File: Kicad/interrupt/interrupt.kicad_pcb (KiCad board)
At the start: 2 copper layers, 68.6 x 53.3 mm, 30 parts, among them IC1 LTC1050CS8#PBF, J1 Conn_LORA, P1 Power, P2 Analog, P3 Digital, P4 Digital, P5 CONN_01X01, P6 CONN_01X01, P7 CONN_01X01, P8 CONN_01X01, Q1 IRF520, U1 GAZ_TO_5

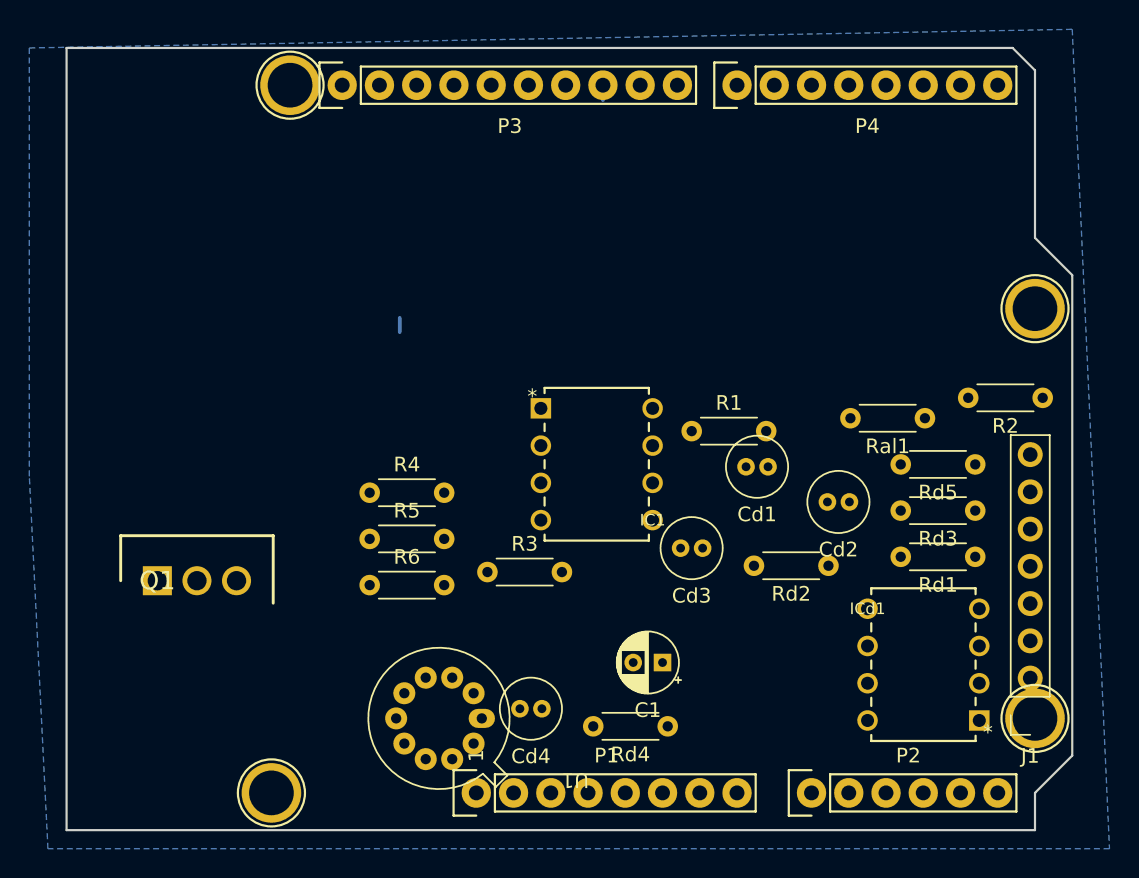
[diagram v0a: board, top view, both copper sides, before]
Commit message: maj
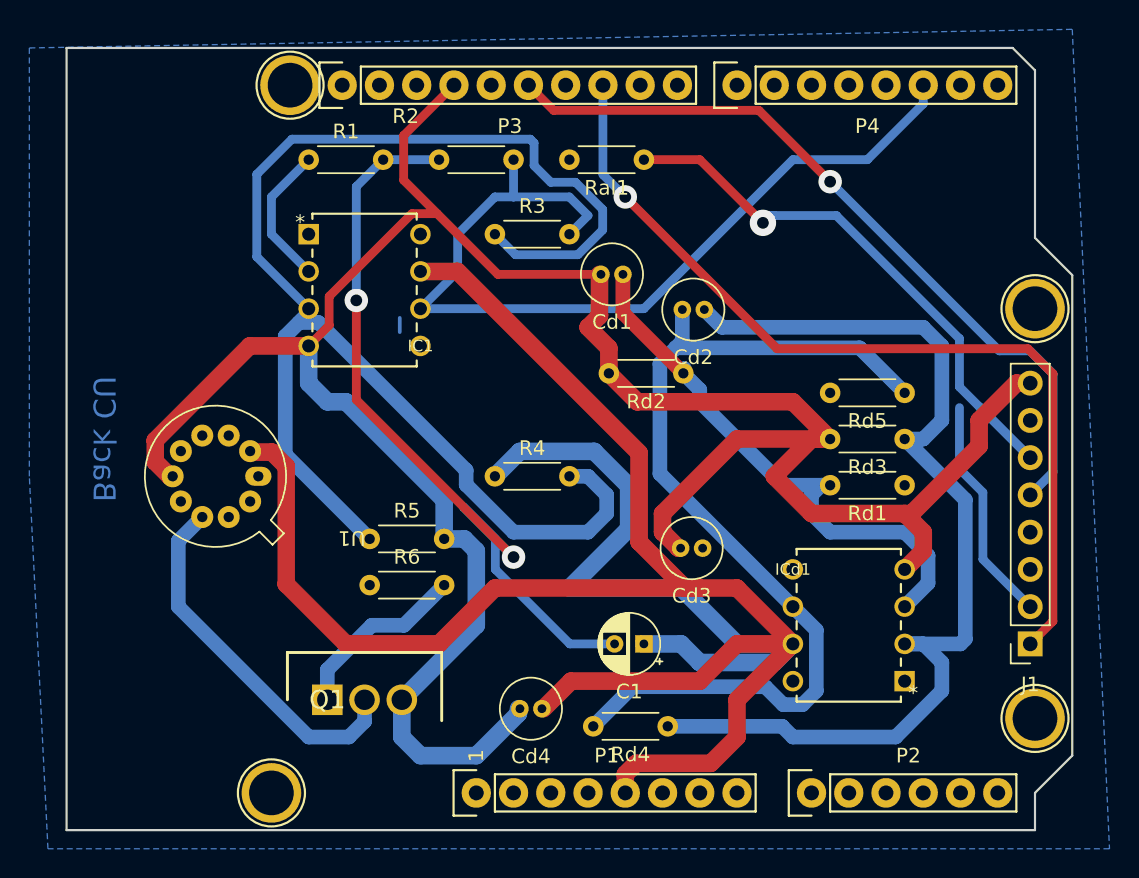
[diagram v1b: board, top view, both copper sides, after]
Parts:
- Q1: footprint IRF520:TO270P460X1020X2008-3P -> KiCadIRF:TO254P465X1024X2050-3P
- moved R2 39.6 mm to (141.5, 80.6)
- moved R1 32.0 mm to (127.5, 80.6)
- moved Ral1 26.0 mm to (150.4, 80.6)
- moved R3 23.0 mm to (140.2, 85.7)
- moved U1 22.5 mm to (122.8, 101.4)
- moved IC1 19.8 mm to (135.1, 93.3)
- moved Cd2 16.4 mm to (154.5, 90.9)
- moved Cd1 16.4 mm to (148.9, 88.5)
- moved Rd2 16.4 mm to (153.1, 95.2)
- moved Q1 14.2 mm to (128.8, 117.5)
- moved R4 8.61 mm to (140.2, 102.2)
- moved Rd3 6.86 mm to (168.1, 99.7)
- moved Rd1 6.86 mm to (168.1, 102.8)
- moved Rd5 6.86 mm to (168.1, 96.5)
- moved ICd1 5.75 mm to (160.5, 108.6)
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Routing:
- net GND: track 0.00 -> 172.8 mm
- net +5V: track 0.00 -> 166.8 mm
- net Net-(IC1-Pad3): track 0.00 -> 99.2 mm
- net Net-(Cd2-Pad1): track 0.00 -> 70.3 mm
- net Net-(Cd2-Pad2): track 0.00 -> 65.2 mm
- net /VAOP: track 0.00 -> 62.3 mm
- net /TX: track 1.99 -> 61.5 mm, vias 0 -> 1
- net Net-(C1-Pad2): track 0.00 -> 56.4 mm, vias 0 -> 2
- net /RST: track 0.00 -> 52.8 mm, vias 0 -> 1
- net +3V3: track 0.00 -> 42.0 mm, vias 0 -> 1
- net Net-(Cd1-Pad1): track 0.00 -> 38.6 mm
- net /GND_Gaz: track 0.00 -> 25.1 mm
- net /RX: track 0.00 -> 15.6 mm
- net Net-(Q1-Pad1): track 0.00 -> 12.4 mm
- net Net-(IC1-Pad2): track 0.00 -> 9.72 mm
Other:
- board text added: "Back CU"
